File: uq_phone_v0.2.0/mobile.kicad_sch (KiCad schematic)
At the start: 25 parts, among them J10 513382474, J11 513382474, J4 20279-001E-03, J5 20279-001E-03, U4 WP SNAP-IN BASE_6000636

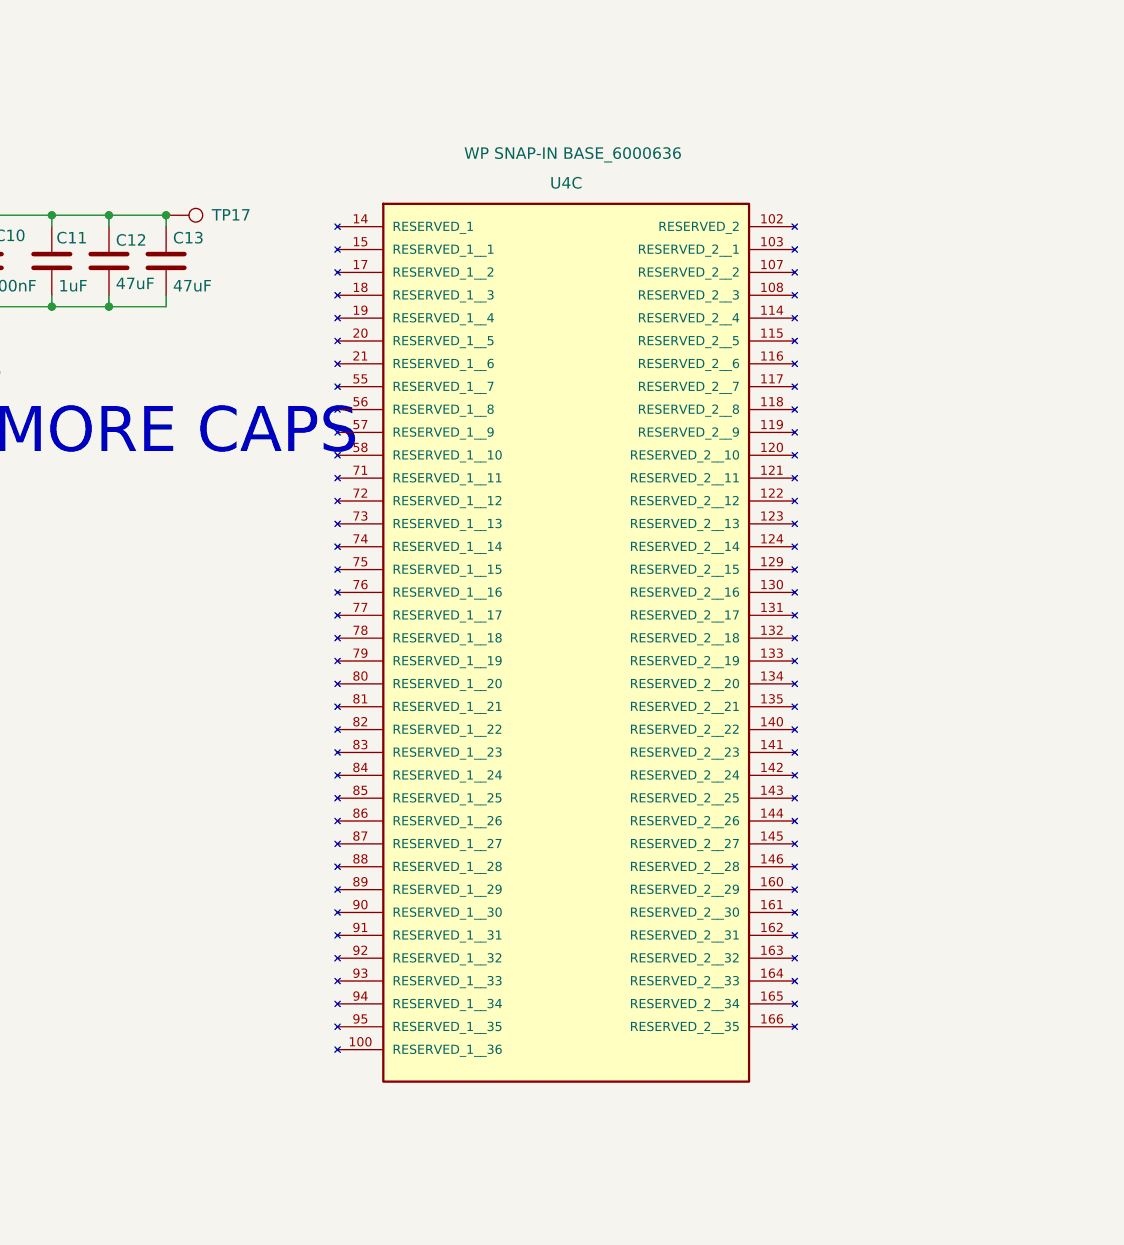
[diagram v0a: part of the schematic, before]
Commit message: Another day of routing and adding components
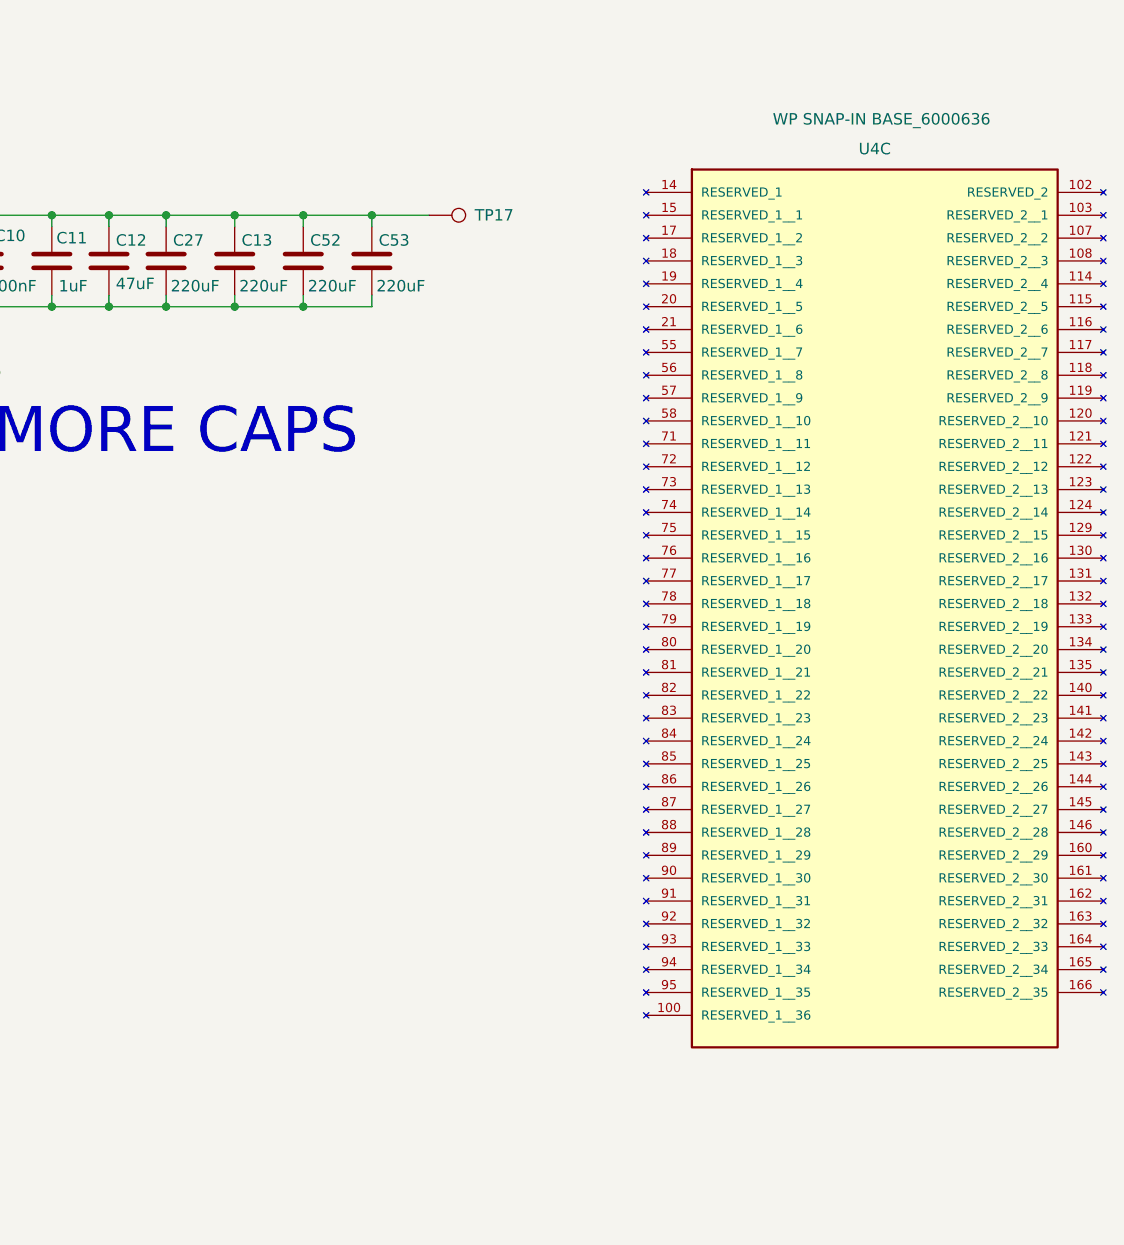
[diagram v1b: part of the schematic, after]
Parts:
- removed C13: 47uF, Capacitor_SMD:C_0805_2012Metric, symbol Capacitors:Capacitor_47uF
- added C13, C27, C52, C53: 220uF, Capacitor_SMD:C_1206_3216Metric, symbol Capacitors:Capacitor_220uF
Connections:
- net GND: now also C13.2, C27.2, C52.2, C53.2
- net VBAT: now also C13.1, C27.1, C52.1, C53.1
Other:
- moved on the sheet: TP17, U4C
